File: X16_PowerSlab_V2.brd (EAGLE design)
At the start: 100 x 80 mm, 40 parts, among them J1 CONN_796636-3, J2 CONN_796636-3, J3 CONN_ET60T

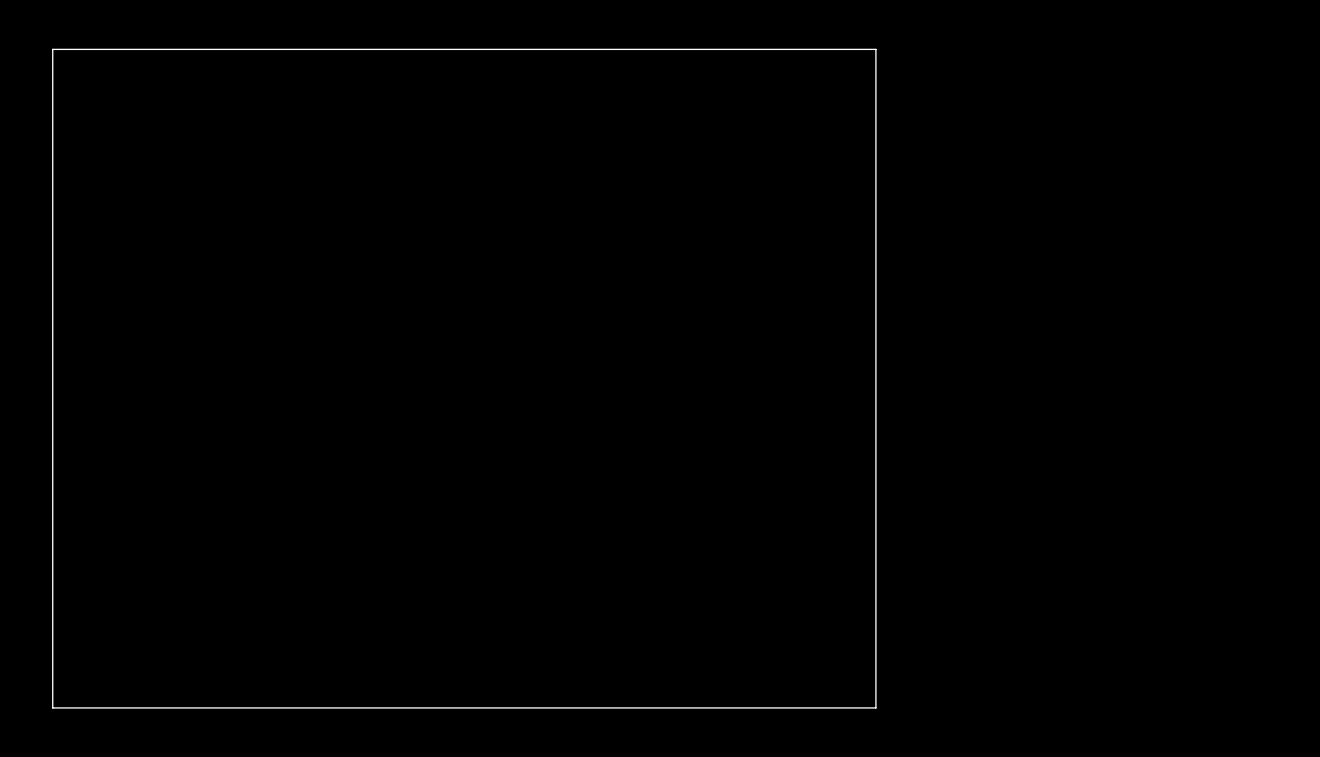
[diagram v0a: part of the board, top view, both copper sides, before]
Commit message: Fixed area of board
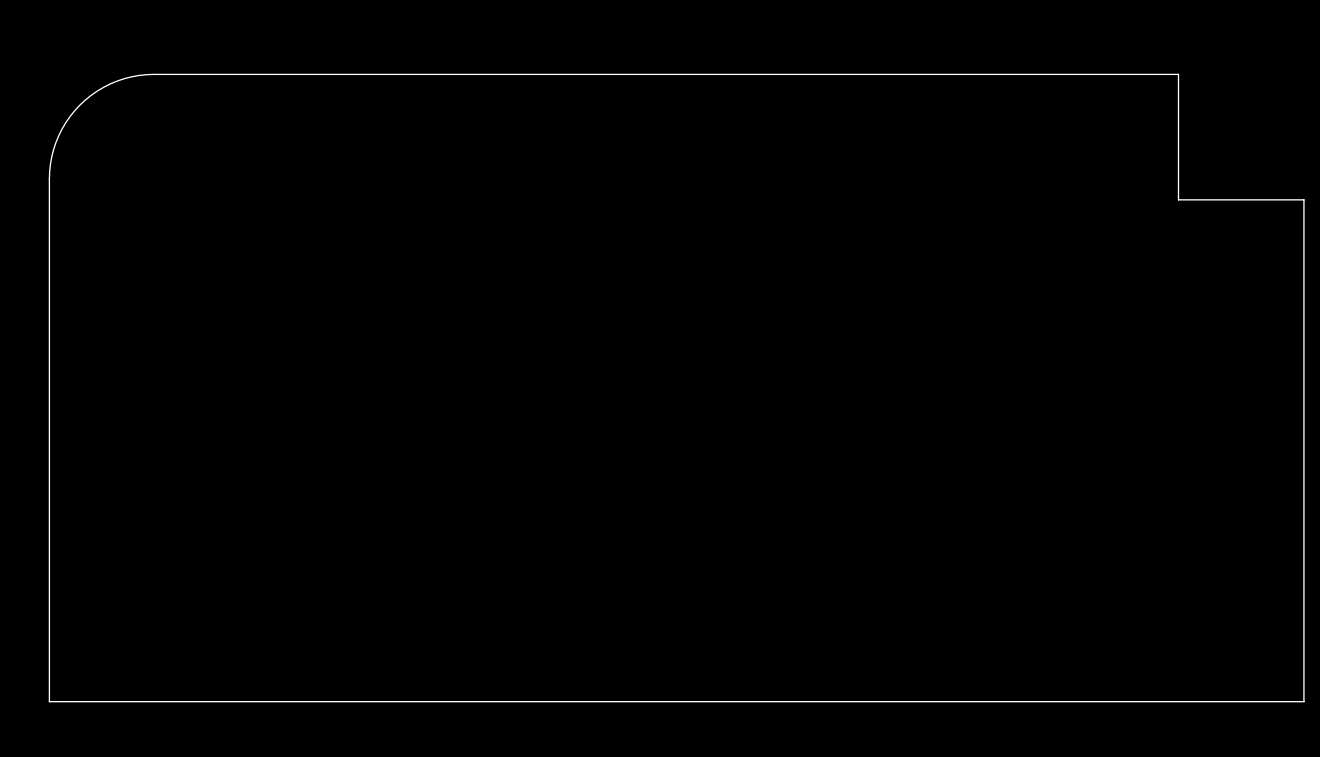
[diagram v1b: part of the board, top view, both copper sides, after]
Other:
- board size 100 x 80 mm -> 152.4 x 76.2 mm
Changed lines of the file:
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@@
 <board>
 <plain>
-<wire x1="0" y1="0" x2="100" y2="0" width="0" layer="20"/>
-<wire x1="100" y1="0" x2="100" y2="80" width="0" layer="20"/>
-<wire x1="100" y1="80" x2="0" y2="80" width="0" layer="20"/>
-<wire x1="0" y1="80" x2="0" y2="0" width="0" layer="20"/>
+<wire x1="-0.4064" y1="0.762" x2="151.9936" y2="0.762" width="0" layer="20"/>
+<wire x1="151.9936" y1="0.762" x2="151.9936" y2="61.722" width="0" layer="20"/>
+<wire x1="-0.4064" y1="64.262" x2="-0.4064" y2="0.762" width="0" layer="20"/>
+<wire x1="136.7536" y1="76.962" x2="136.7536" y2="61.722" width="0" layer="20"/>
+<wire x1="136.7536" y1="61.722" x2="151.9936" y2="61.722" width="0" layer="20"/>
+<wire x1="12.2936" y1="76.962" x2="136.7536" y2="76.962" width="0" layer="20"/>
+<wire x1="12.2936" y1="76.962" x2="-0.4064" y2="64.262" width="0" layer="20" curve="90"/>
 </plain>
 <attributes>

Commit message: Started placing components on board
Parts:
- moved U$3 381.9 mm to (73.7, 58.4), turned to 180 degrees
- moved J3 164.1 mm to (67.3, 8.89)
- moved U$1 137.2 mm to (12.7, 10.2), turned to 180 degrees
- moved J2 98.3 mm to (6.35, 22.9), turned to 90 degrees
- moved J1 48.4 mm to (6.35, 43.2), turned to 90 degrees
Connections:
- removed net 5.2V: 5V_TEST.1, COUT1.+, COUT2.+, COUT3.+, L1.2, R2.2, R6.1, U$4.5.2V
- net 5V: now also 5V_TEST.1, COUT1.+, COUT2.+, COUT3.+, L1.2, R2.2, R6.1, U$4.5.2V
